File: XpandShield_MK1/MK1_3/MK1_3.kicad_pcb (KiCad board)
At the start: 2 copper layers, 53.3 x 101.6 mm, 1 part

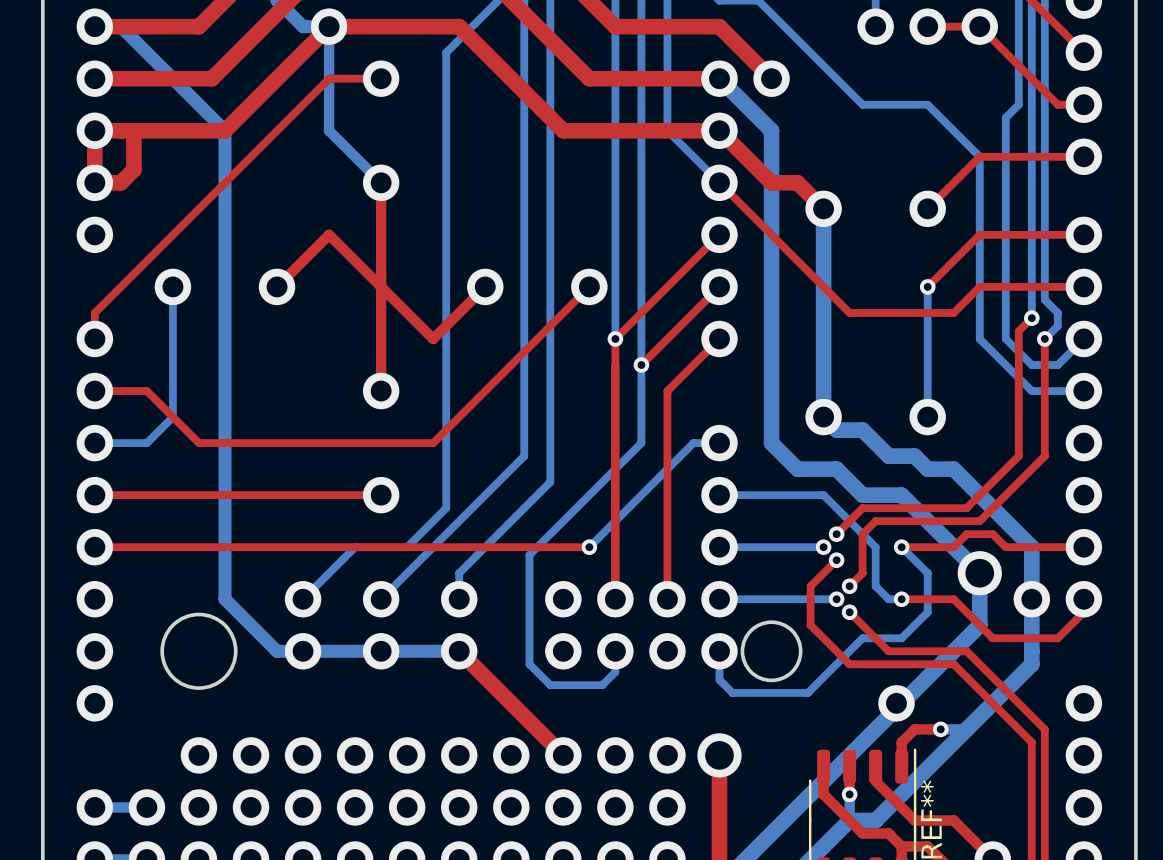
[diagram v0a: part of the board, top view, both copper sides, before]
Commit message: Updated MK1 PCBs
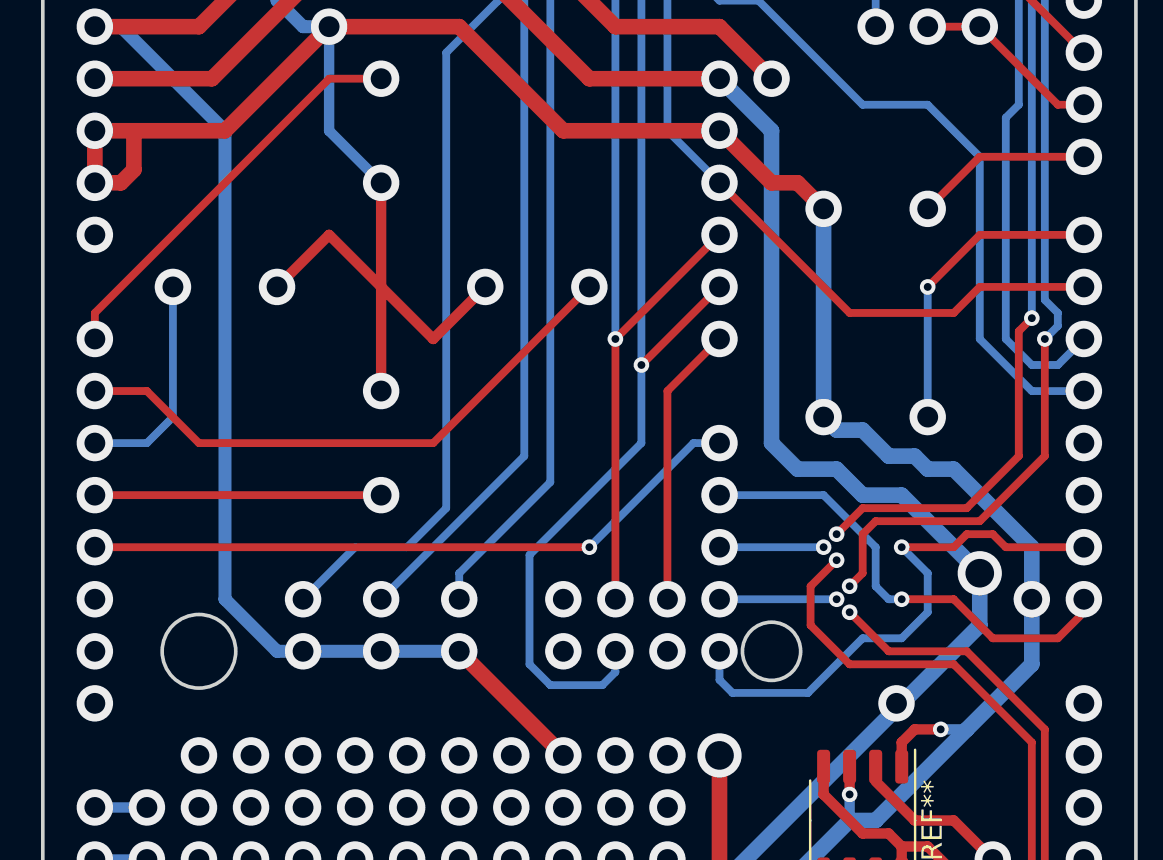
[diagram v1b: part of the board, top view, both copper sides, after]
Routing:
- net (no net): track 1616.6 -> 1605.2 mm

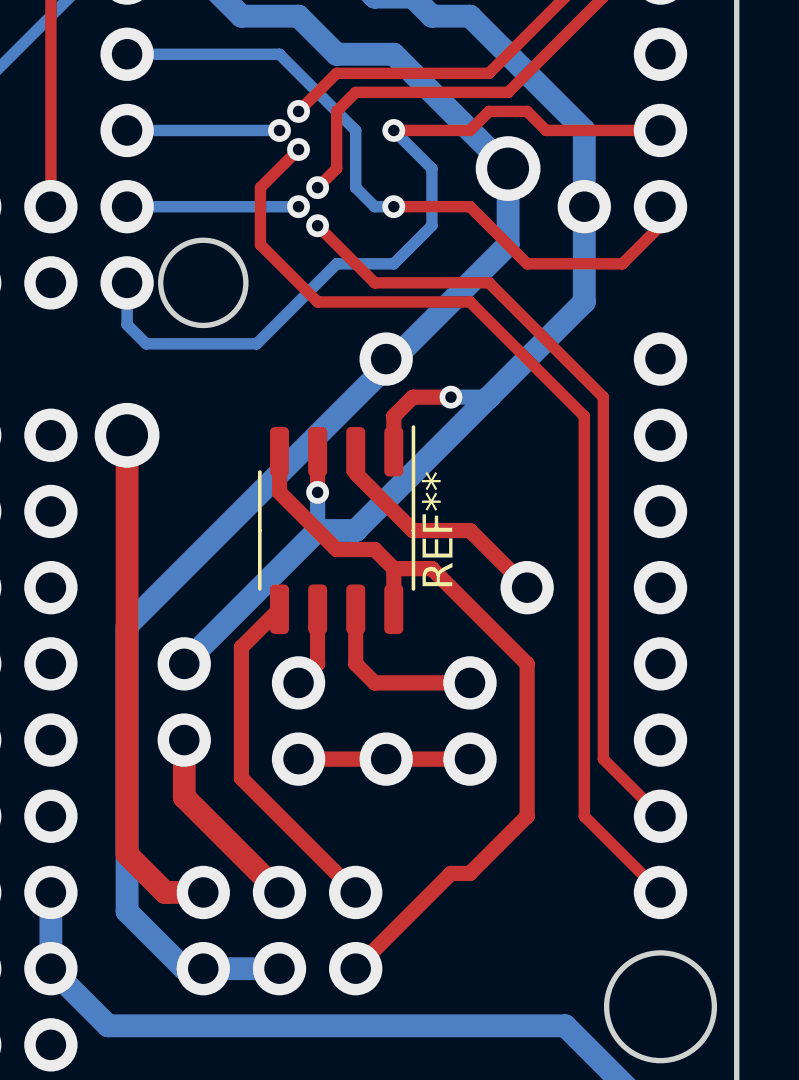
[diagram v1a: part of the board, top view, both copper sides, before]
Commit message: Updated MK1_3 board
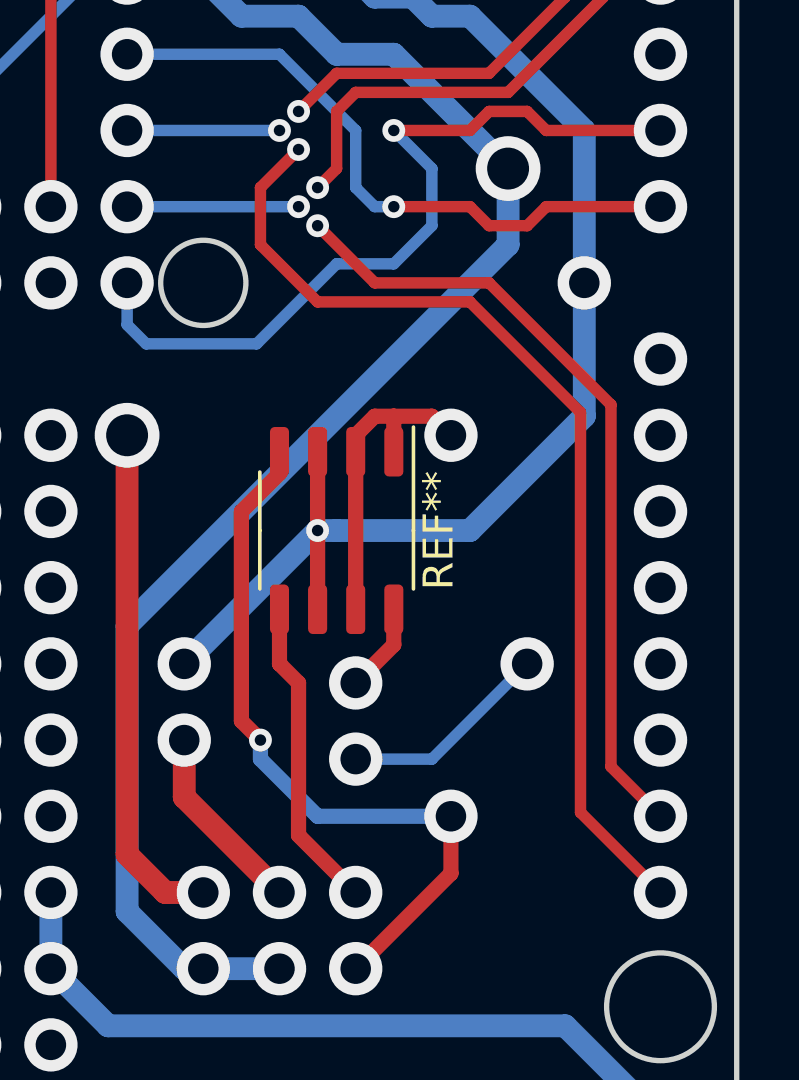
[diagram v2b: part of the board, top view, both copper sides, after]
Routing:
- net (no net): track 1605.2 -> 1600.9 mm, vias 283 -> 281

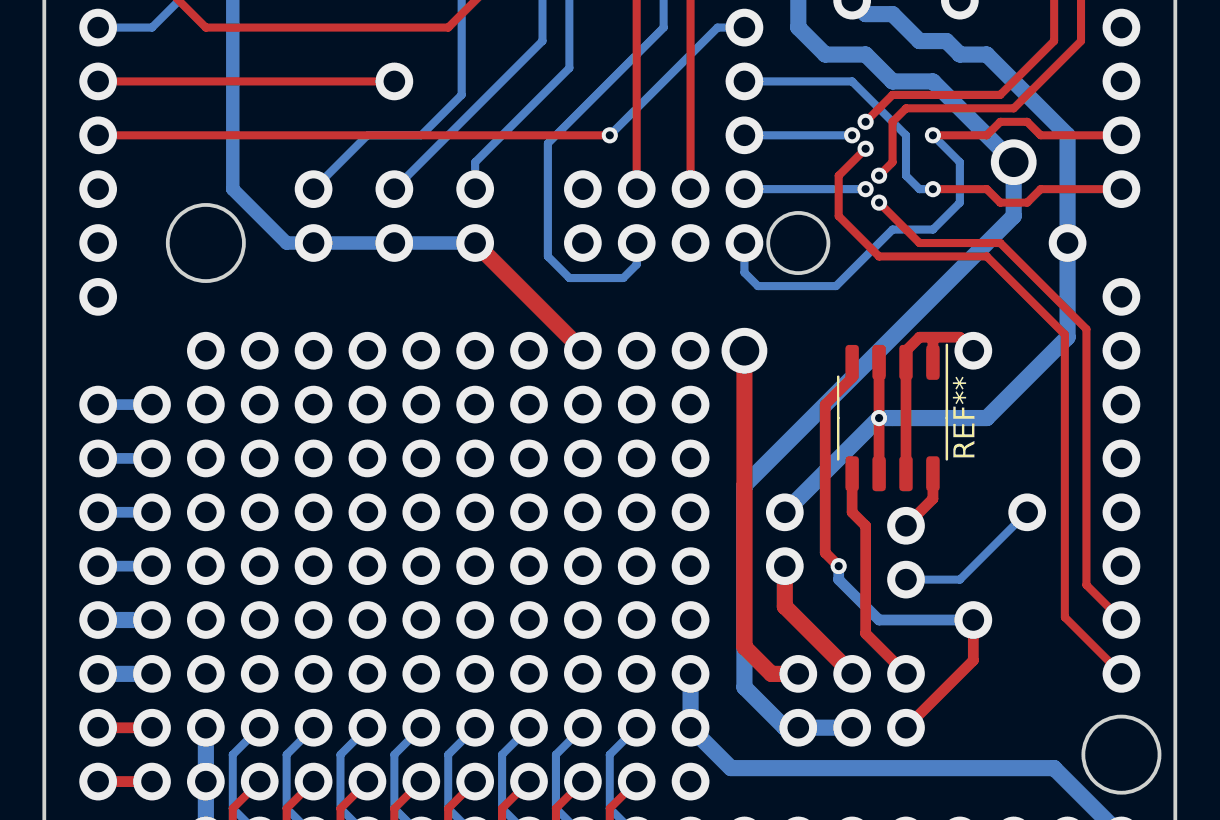
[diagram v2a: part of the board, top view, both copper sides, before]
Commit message: Updated MK1_3 Design
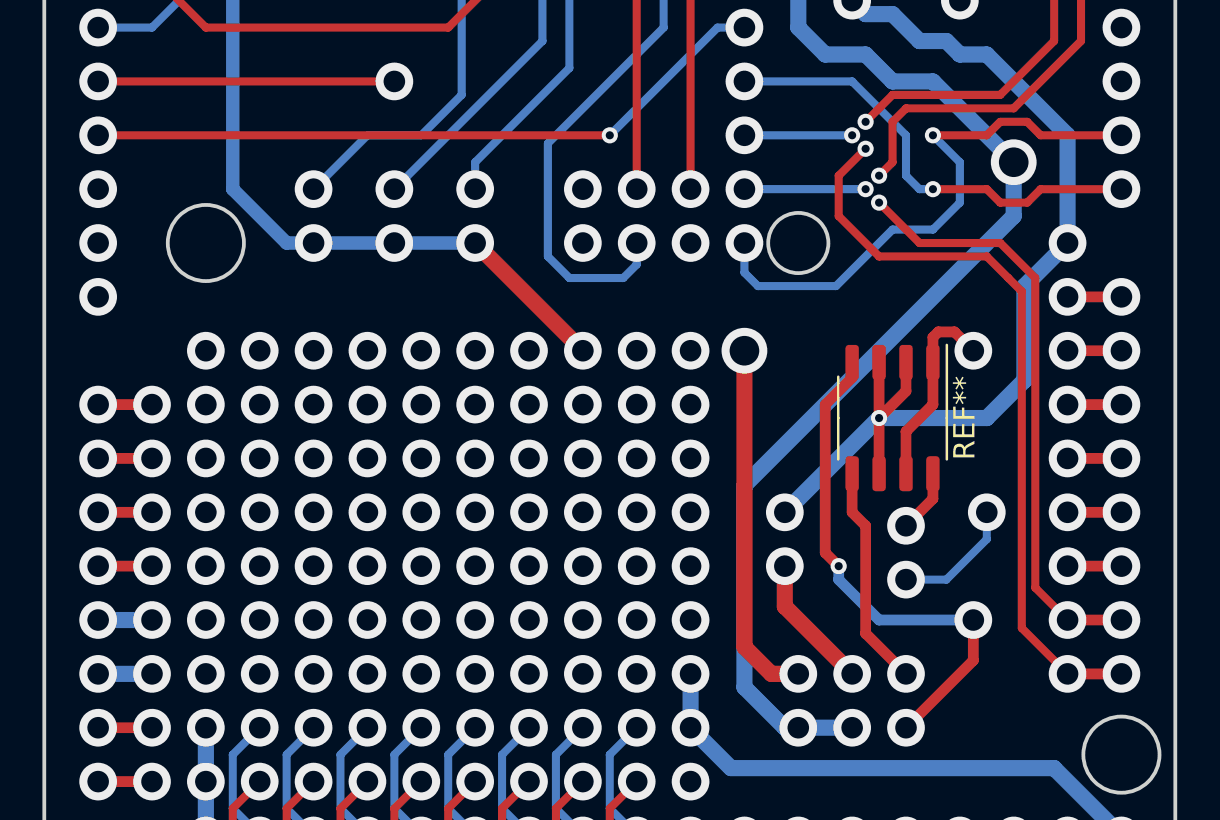
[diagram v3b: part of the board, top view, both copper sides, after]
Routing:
- net (no net): track 1600.9 -> 1619.7 mm, vias 281 -> 289
